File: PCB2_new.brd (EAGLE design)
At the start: 100 x 80 mm, 113 parts

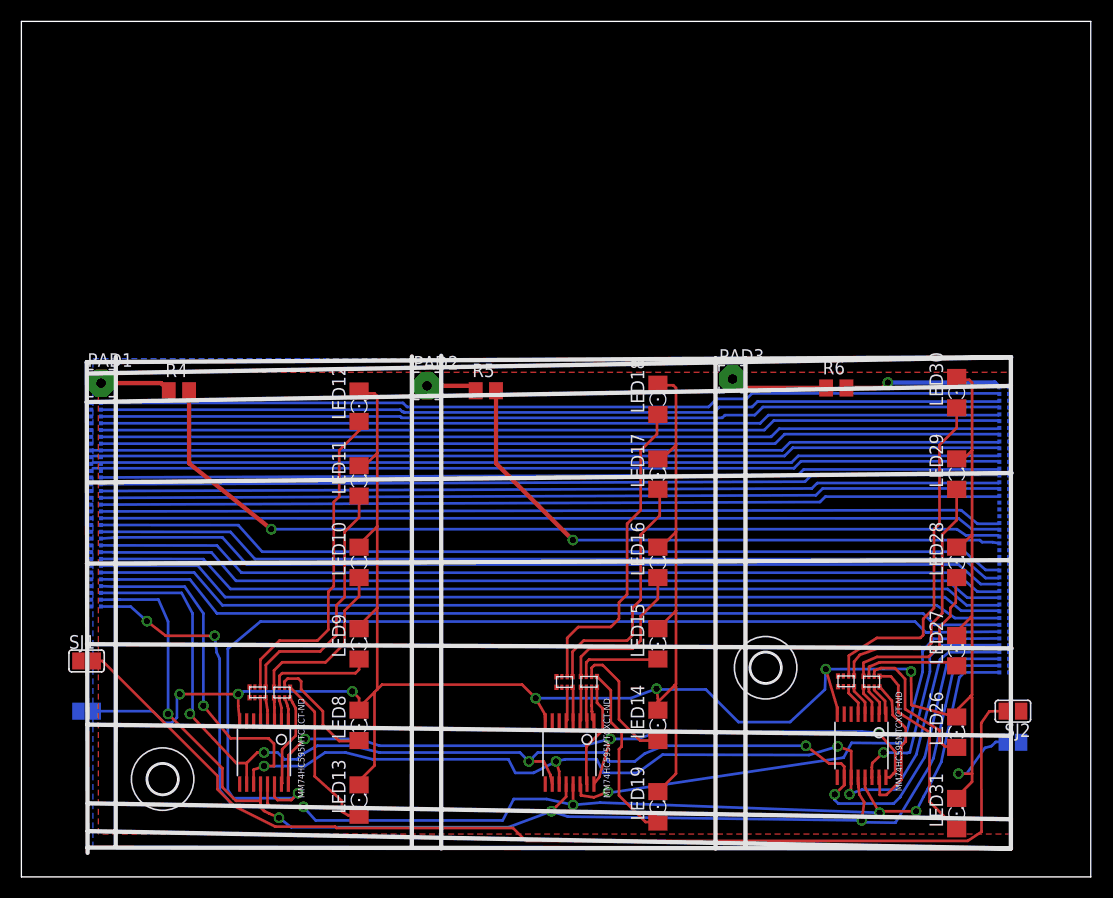
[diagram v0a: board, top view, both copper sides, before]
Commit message: Finished PCB4. Finished gerbers for PCB1, 2, 3, and 4
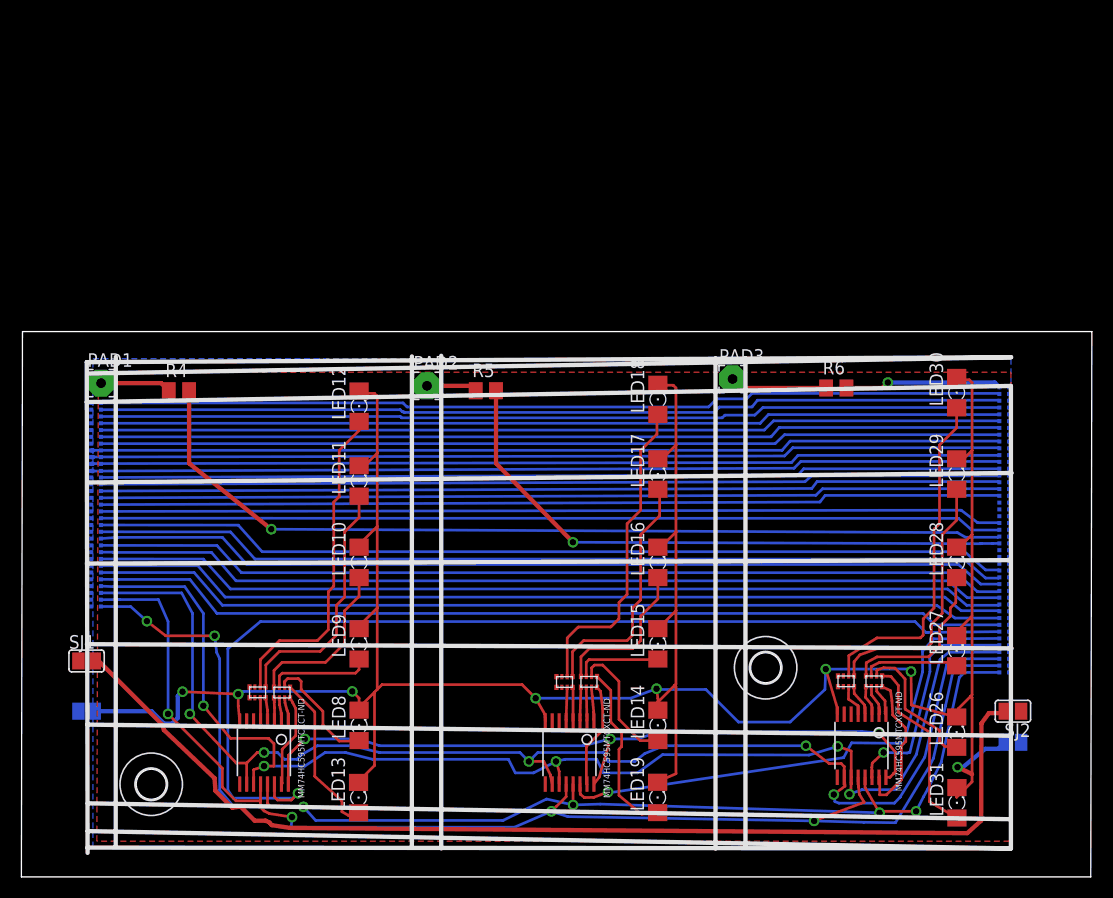
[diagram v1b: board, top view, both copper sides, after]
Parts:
- moved H1 1.17 mm to (12.1, 8.66)
- moved LED31 1.02 mm to (87.5, 6.93)
- moved LED19 0.88 mm to (59.5, 7.43)
- moved LED13 0.23 mm to (31.5, 7.41)
- moved U$78 0.23 mm to (79.7, 18.3)
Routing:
- net RCK: track 119.1 -> 123.1 mm
- net VDD: track 103.5 -> 102.3 mm
- net N$67: track 18.2 -> 17.4 mm
- net G: track 122.0 -> 121.3 mm
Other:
- board size 100 x 80 mm -> 100.1 x 51 mm
